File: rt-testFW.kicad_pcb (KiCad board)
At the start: 2 copper layers, 77 x 55 mm, 11 parts, among them J1-1Min1 Conn_01x02_Male, J2-2Min1 Conn_01x02_Male, J3-3Min1 Conn_01x02_Male, J4-5Min1 Conn_01x02_Male

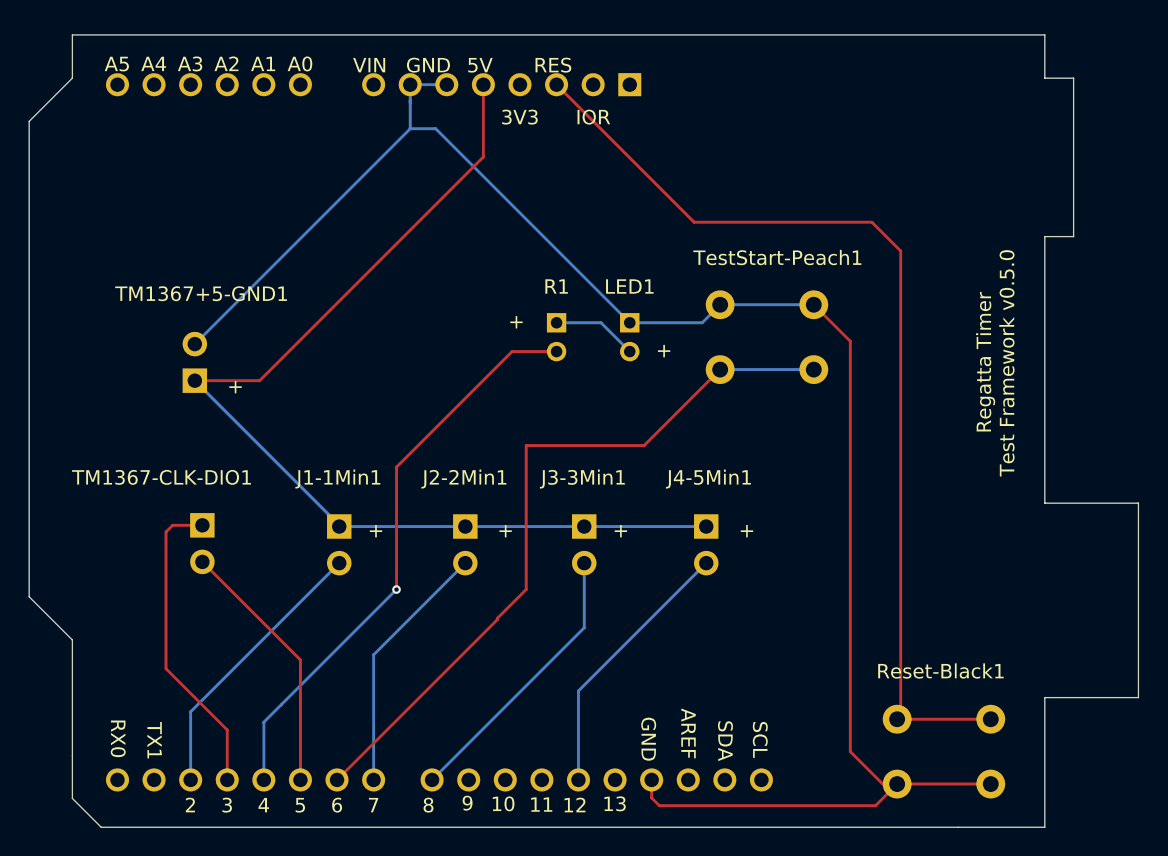
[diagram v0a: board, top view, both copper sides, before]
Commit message: pcb relayout complete
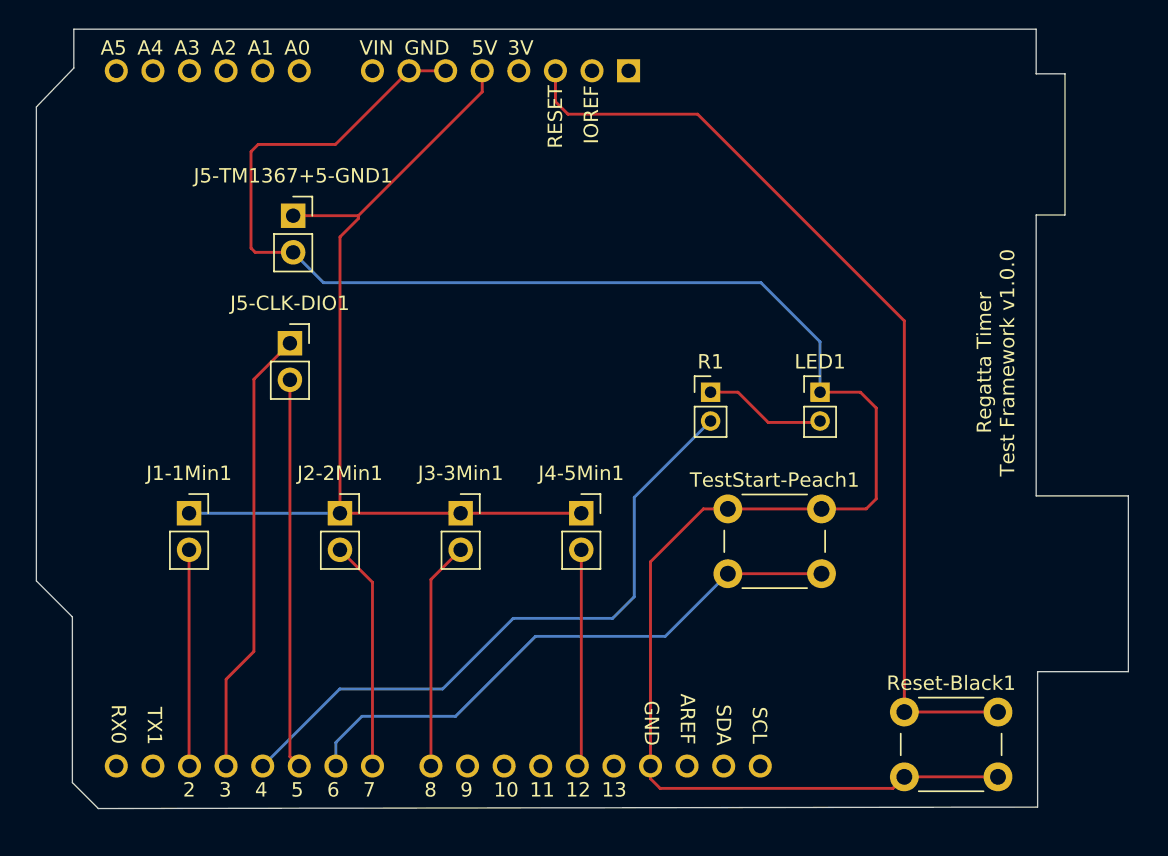
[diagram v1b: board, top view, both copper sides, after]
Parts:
- removed TM1367+5-GND1, TM1367-CLK-DIO1: Conn_01x02_Male, Connector_PinSocket_2.54mm:PinSocket_1x02_P2.54mm_Vertical
- added J5-CLK-DIO1: Conn_01x02_Male, Connector_PinSocket_2.54mm:PinSocket_1x02_P2.54mm_Vertical, F.Cu at (177.1, 94.4)
- added J5-TM1367+5-GND1: Conn_01x02_Male, Connector_PinSocket_2.54mm:PinSocket_1x02_P2.54mm_Vertical, F.Cu at (177.3, 85.5)
- A1, J1-1Min1, J2-2Min1, J3-3Min1, J4-5Min1, LED1, R1, Reset-Black1, TestStart-Peach1: moved to F.Cu
- moved TestStart-Peach1 15.4 mm to (207.5, 105.9), turned to 0 degrees
- moved LED1 14.1 mm to (213.9, 97.8), turned to 0 degrees
- moved R1 11.7 mm to (206.3, 97.8), turned to 0 degrees
- moved J1-1Min1 10.5 mm to (170.1, 106.2), turned to 0 degrees
- moved J2-2Min1 8.75 mm to (180.6, 106.2), turned to 0 degrees
- moved J4-5Min1 8.72 mm to (197.3, 106.2), turned to 0 degrees
- moved J3-3Min1 8.63 mm to (188.9, 106.2), turned to 0 degrees
- moved Reset-Black1 6.02 mm to (219.8, 120.0), turned to 0 degrees
- moved A1 0.97 mm to (200.6, 75.5), turned to 0 degrees
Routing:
- net GND: track 123.0 -> 136.2 mm
- net Net-(A1-D6): track 50.8 -> 40.2 mm
- net Net-(A1-D3): track 21.7 -> 31.2 mm
- net Net-(A1-D5): track 18.0 -> 27.1 mm
- net Net-(A1-D4): track 40.0 -> 45.1 mm, vias 1 -> 0
- net +5V: track 71.2 -> 66.6 mm
- net Net-(A1-D2): track 19.3 -> 15.0 mm
- net Net-(A1-D12): track 18.7 -> 15.1 mm
- net Net-(A1-D8): track 19.4 -> 15.9 mm
- net Net-(LED1-A): track 5.91 -> 8.51 mm
- net Net-(A1-D7): track 17.7 -> 15.9 mm
- net Net-(A1-~{RESET}): track 67.8 -> 66.3 mm
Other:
- board size 77 x 55 mm -> 75.8 x 54.1 mm
- board text added: "Regatta Timer Test Framework v1.0.0"
- board text removed: "+"
- board text removed: "10"
- board text removed: "11"
- board text removed: "12"
- board text removed: "13"
- board text removed: "2"
- board text removed: "3"
- board text removed: "3V3"
- board text removed: "4"
- board text removed: "5"
- board text removed: "5V"
- board text removed: "6"
- board text removed: "7"
- board text removed: "8"
- board text removed: "9"
- board text removed: "A0"
- board text removed: "A1"
- board text removed: "A2"
- board text removed: "A3"
- board text removed: "A4"
- board text removed: "A5"
- board text removed: "AREF"
- board text removed: "GND"
- board text removed: "IOR"
- board text removed: "RES"
- board text removed: "RX0"
- board text removed: "Regatta Timer Test Framework v0.5.0"
- board text removed: "SCL"
- board text removed: "SDA"
- board text removed: "TX1"
- board text removed: "VIN"
